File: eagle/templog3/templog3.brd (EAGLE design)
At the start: 31.2 x 16 mm, 25 parts, among them IC1 MCP170312MB, J2 3-PIN SMD, U1 ATSAMD21G-A, X2 ZX62D-B-5PA8, Y2 32.768kHz

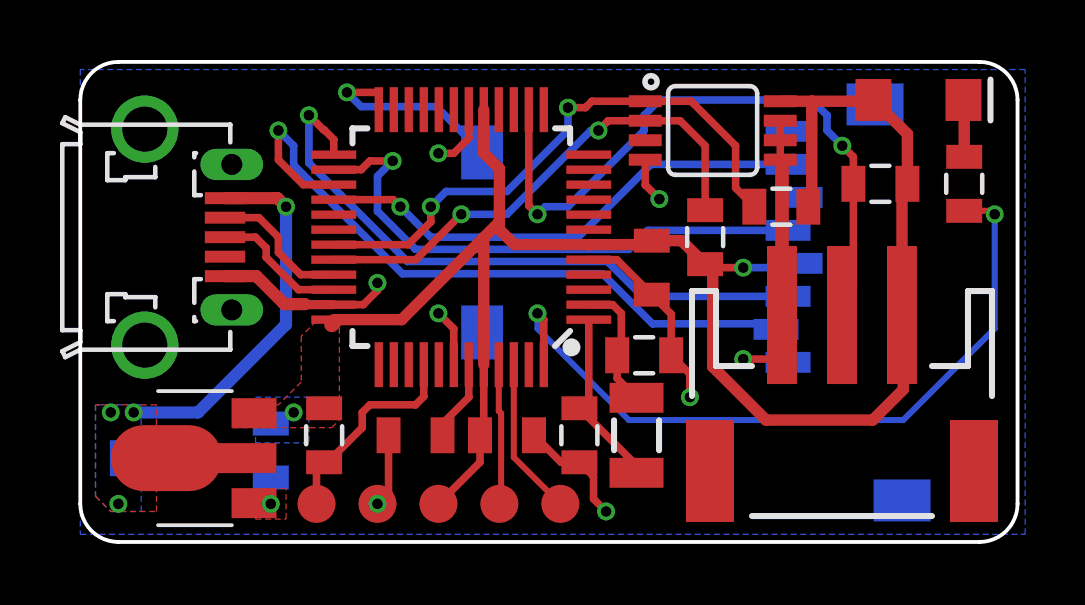
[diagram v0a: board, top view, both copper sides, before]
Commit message: batteryholder boards minor changes
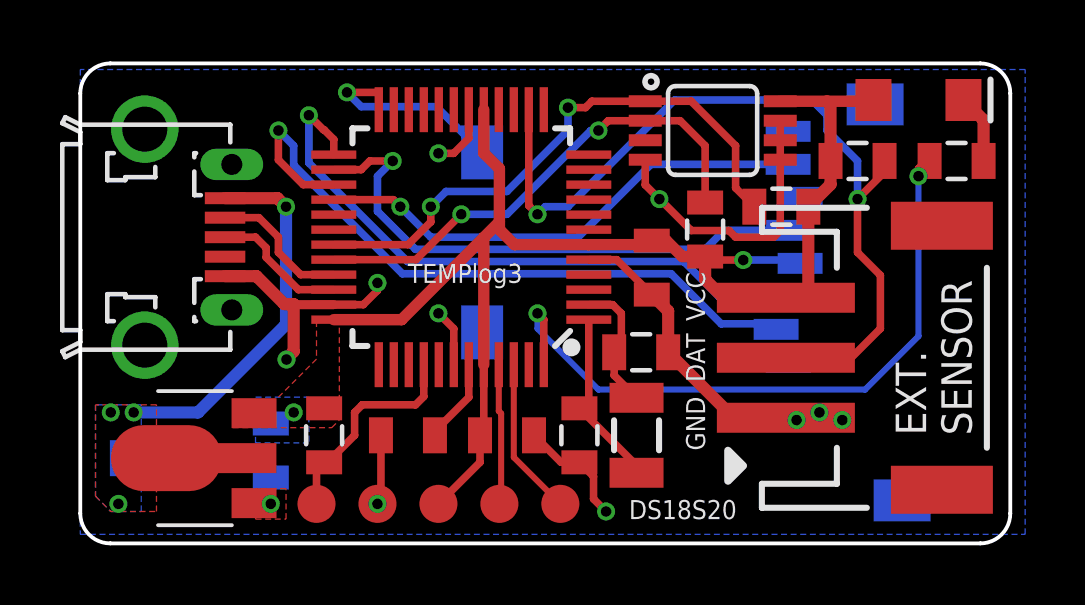
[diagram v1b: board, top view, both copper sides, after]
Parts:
- moved J2 4.43 mm to (28.3, 9.20), turned to 270 degrees
- moved R_I2C_3 1.08 mm to (25.9, 15.7), turned to 180 degrees
- moved R_I2C_4 0.80 mm to (29.2, 15.7), turned to 180 degrees
- moved C6 0.25 mm to (10.9, 6.60)
- moved R_I2C_1 0.25 mm to (20.8, 13.5)
- moved C5 0.14 mm to (18.7, 9.37)
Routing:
- net VCC: track 59.8 -> 45.6 mm
- net EXT_SENSOR: track 22.5 -> 28.1 mm
- net GND: track 34.0 -> 38.0 mm, vias 9 -> 11
- net LED: track 24.9 -> 22.6 mm
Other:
- board size 31.2 x 16 mm -> 31 x 16 mm
- board text added: "DAT"
- board text added: "DS18S20"
- board text added: "EXT."
- board text added: "GND"
- board text added: "SENSOR"
- board text added: "VCC"
